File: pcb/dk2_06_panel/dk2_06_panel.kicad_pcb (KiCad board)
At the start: 2 copper layers, 121.9 x 128.5 mm, 51 parts

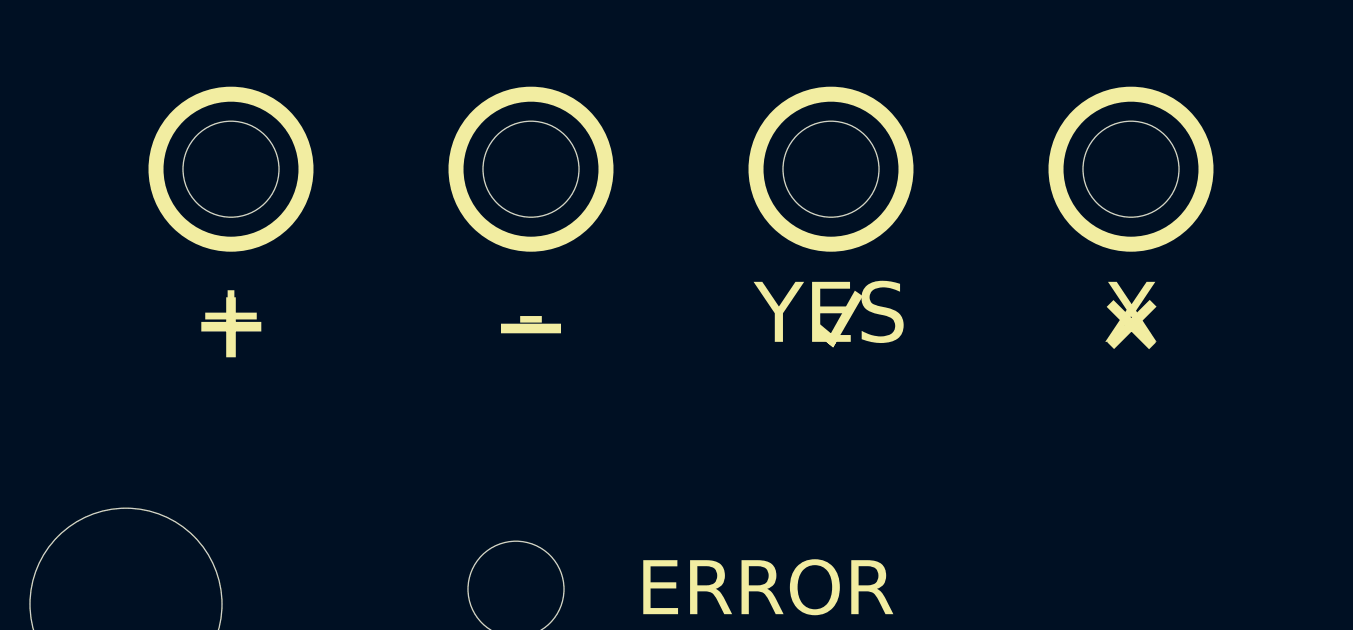
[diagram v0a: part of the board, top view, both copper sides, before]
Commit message: getting back into development...
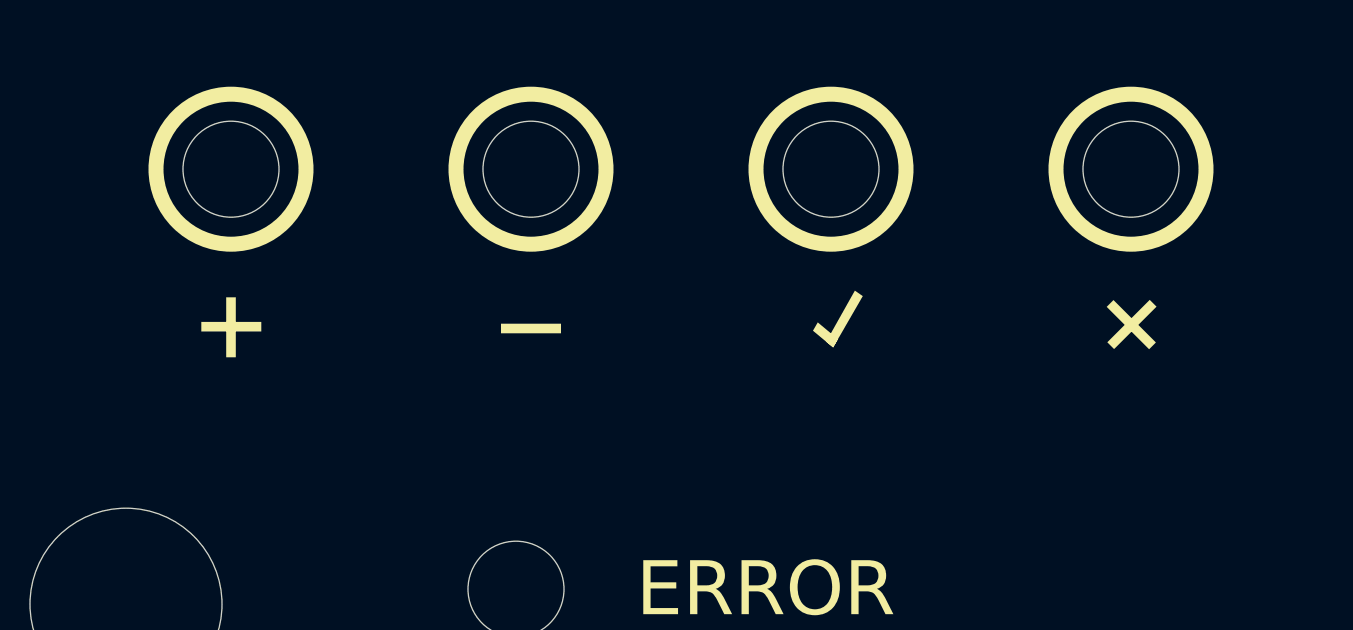
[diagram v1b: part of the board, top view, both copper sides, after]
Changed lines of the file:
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@@
 			(layer "F.CrtYd")
 		)
-		(fp_text user "${VALUE}"
-			(at 0 6 0)
-			(unlocked yes)
-			(layer "F.SilkS")
-			(effects
-				(font
-					(face "Consolas")
-					(size 2 2)
-					(thickness 0.15)
-				)
-				(justify bottom)
-			)
-			(render_cache "-" 0
-				(polygon
-					(pts
-						(xy 157.908863 114.526922) (xy 157.09187 114.526922) (xy 157.09187 114.302219) (xy 157.908863 114.302219)
-					)
-				)
-			)
-		)
 		(fp_text user "${REFERENCE}"
 			(at 0 0.45 0)
@@
 			(layer "F.CrtYd")
 		)
-		(fp_text user "${VALUE}"
-			(at 0 6 0)
-			(unlocked yes)
-			(layer "F.SilkS")
-			(effects
-				(font
-					(face "Consolas")
-					(size 2 2)
-					(thickness 0.15)
-				)
-				(justify bottom)
-			)
-			(render_cache "X" 0
-				(polygon
-					(pts
-						(xy 178.236759 115.16) (xy 177.929257 115.16) (xy 177.494871 114.438628) (xy 177.05902 115.16)
-						(xy 176.75567 115.16) (xy 177.350035 114.249218) (xy 176.803542 113.378004) (xy 177.09187 113.378004)
-						(xy 177.500366 114.05016) (xy 177.911549 113.378004) (xy 178.191574 113.378004) (xy 177.643737 114.238349)
-					)
-				)
-			)
-		)
 		(fp_text user "${REFERENCE}"
 			(at 0 0.45 0)
@@
 			(layer "F.CrtYd")
 		)
-		(fp_text user "${VALUE}"
-			(at 0 6 0)
-			(unlocked yes)
-			(layer "F.SilkS")
-			(effects
-				(font
-					(face "Consolas")
-					(size 2 2)
-					(thickness 0.15)
-				)
-				(justify bottom)
-			)
-			(render_cache "YES" 0
-				(polygon
-					(pts
-						(xy 166.731734 113.378004) (xy 166.085467 114.524602) (xy 166.085467 115.16) (xy 165.839637 115.16)
-						(xy 165.839637 114.519106) (xy 165.193371 113.378004) (xy 165.487073 113.378004) (xy 165.842324 114.030498)
-						(xy 165.973482 114.292571) (xy 166.093772 114.055045) (xy 166.453053 113.378004)
-					)
-				)
-				(polygon
-					(pts
-						(xy 168.020848 115.16) (xy 167.005775 115.16) (xy 167.005775 113.378004) (xy 168.020848 113.378004)
-						(xy 168.020848 113.583168) (xy 167.248918 113.583168) (xy 167.248918 114.13418) (xy 167.990806 114.13418)
-						(xy 167.990806 114.339344) (xy 167.248918 114.339344) (xy 167.248918 114.952882) (xy 168.020848 114.952882)
-					)
-				)
-				(polygon
-					(pts
-						(xy 169.631019 114.674689) (xy 169.617534 114.796228) (xy 169.579117 114.897683) (xy 169.517264 114.984968)
-						(xy 169.434281 115.056929) (xy 169.334408 115.11147) (xy 169.210799 115.152062) (xy 169.076599 115.175282)
-						(xy 168.923325 115.183447) (xy 168.781909 115.177951) (xy 168.646598 115.164274) (xy 168.524354 115.145223)
-						(xy 168.420551 115.121898) (xy 168.420551 114.88657) (xy 168.526792 114.920037) (xy 168.65075 114.946653)
-						(xy 168.782847 114.962716) (xy 168.941033 114.968513) (xy 169.05413 114.963495) (xy 169.14119 114.950073)
-						(xy 169.218821 114.926201) (xy 169.2765 114.895484) (xy 169.322464 114.854687) (xy 169.352948 114.807313)
-						(xy 169.370666 114.752718) (xy 169.376884 114.688367) (xy 169.366532 114.620327) (xy 169.336584 114.564658)
-						(xy 169.291059 114.517065) (xy 169.230705 114.473066) (xy 169.162075 114.435157) (xy 169.081106 114.399183)
-						(xy 168.909648 114.330062) (xy 168.738189 114.252882) (xy 168.658065 114.206889) (xy 168.58859 114.15433)
-						(xy 168.529315 114.092577) (xy 168.482711 114.020973) (xy 168.45299 113.939469) (xy 168.442411 113.839134)
-						(xy 168.451842 113.748714) (xy 168.480635 113.658517) (xy 168.528782 113.575483) (xy 168.599459 113.500614)
-						(xy 168.688516 113.439801) (xy 168.806455 113.389117) (xy 168.939666 113.358096) (xy 169.107728 113.346741)
-						(xy 169.205426 113.350893) (xy 169.312038 113.362494) (xy 169.418528 113.379713) (xy 169.516225 113.40023)
-						(xy 169.516225 113.619316) (xy 169.305809 113.57352) (xy 169.201365 113.56163) (xy 169.102233 113.557766)
-						(xy 168.96369 113.567151) (xy 168.864391 113.591678) (xy 168.794853 113.627376) (xy 168.739664 113.679854)
-						(xy 168.707562 113.741175) (xy 168.696546 113.814466) (xy 168.70687 113.882642) (xy 168.736846 113.93903)
-						(xy 168.782387 113.987264) (xy 168.842725 114.031964) (xy 168.911402 114.070349) (xy 168.992324 114.106458)
-						(xy 169.163782 114.175579) (xy 169.335241 114.253492) (xy 169.415297 114.300242) (xy 169.484839 114.353998)
-						(xy 169.544085 114.417086) (xy 169.590719 114.490163) (xy 169.620443 114.57299)
-					)
-				)
-			)
-		)
 		(fp_text user "${REFERENCE}"
 			(at 0 0.45 0)
@@
 			(layer "F.CrtYd")
 		)
-		(fp_text user "${VALUE}"
-			(at 0 6 0)
-			(unlocked yes)
-			(layer "F.SilkS")
-			(effects
-				(font
-					(face "Consolas")
-					(size 2 2)
-					(thickness 0.15)
-				)
-				(justify bottom)
-			)
-			(render_cache "+" 0
-				(polygon
-					(pts
-						(xy 148.154693 114.519106) (xy 147.617847 114.519106) (xy 147.617847 115.074026) (xy 147.382763 115.074026)
-						(xy 147.382763 114.519106) (xy 146.845918 114.519106) (xy 146.845918 114.311988) (xy 147.382763 114.311988)
-						(xy 147.382763 113.757069) (xy 147.617847 113.757069) (xy 147.617847 114.311988) (xy 148.154693 114.311988)
-					)
-				)
-			)
-		)
 		(fp_text user "${REFERENCE}"
